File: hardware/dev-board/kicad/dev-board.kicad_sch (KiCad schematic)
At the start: 0 parts

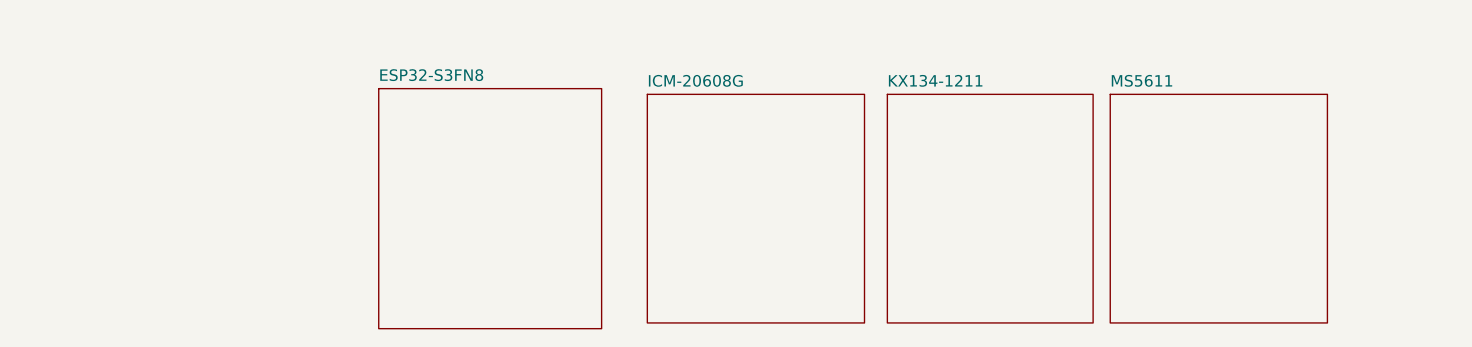
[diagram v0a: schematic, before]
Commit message: Update Files
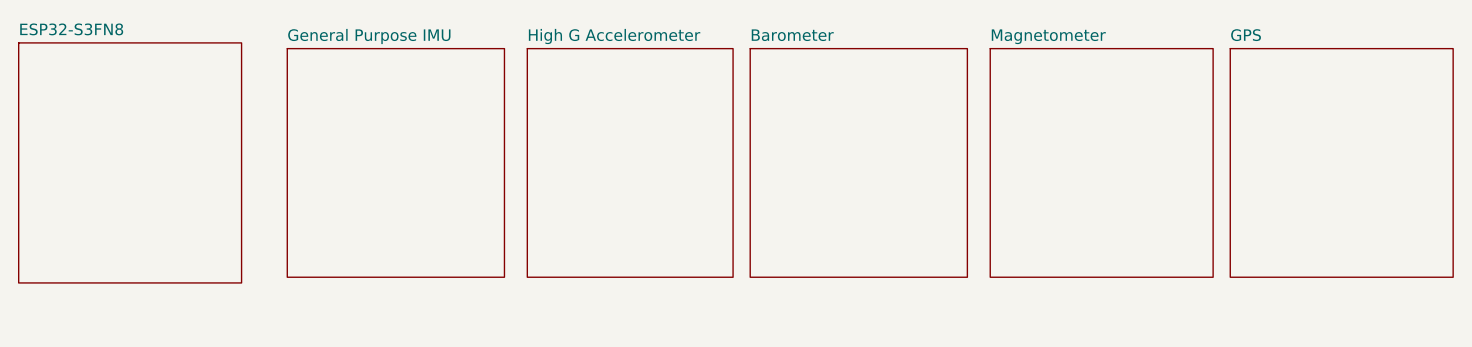
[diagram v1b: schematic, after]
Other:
- sheet ICM-20608G renamed General Purpose IMU
- sheet KX134-1211 renamed High G Accelerometer
- sheet MS5611 renamed Barometer
- added sheet GPS (hierarchical_sheets/zoe-m8q.kicad_sch)
- added sheet Magnetometer (hierarchical_sheets/mmc5983ma.kicad_sch)
